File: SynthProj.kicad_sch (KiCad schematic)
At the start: 29 parts, among them J18 Ext In

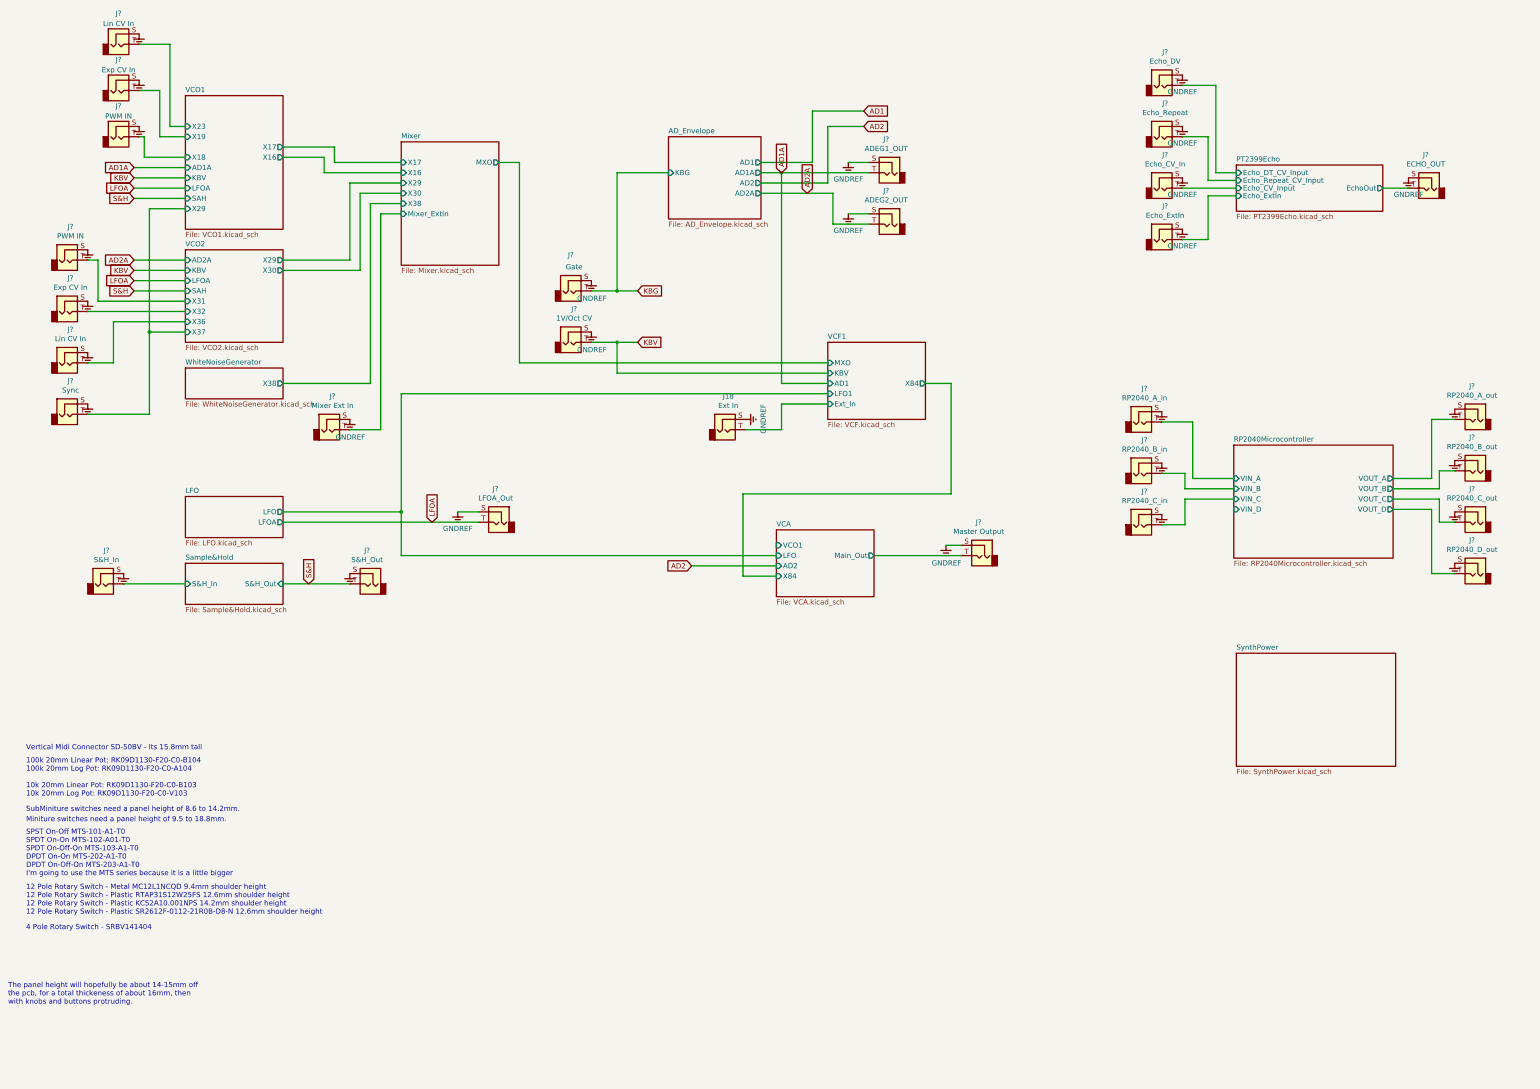
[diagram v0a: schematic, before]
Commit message: more routing...
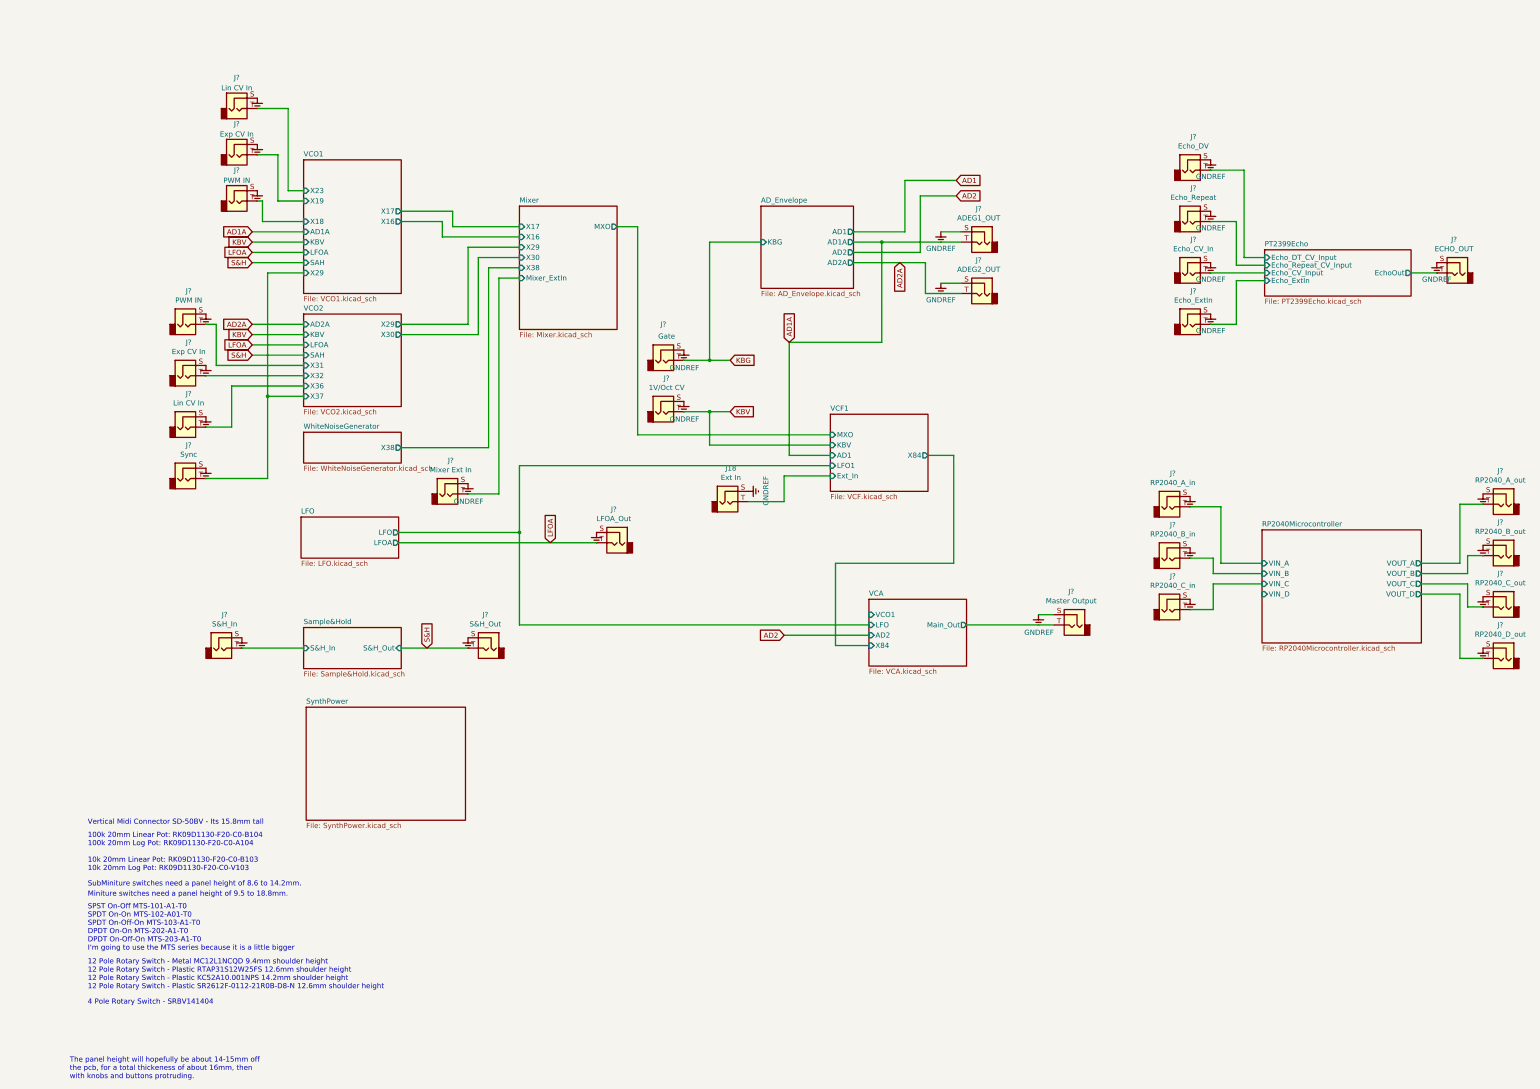
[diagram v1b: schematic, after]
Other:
- moved on the sheet: J18, J?
